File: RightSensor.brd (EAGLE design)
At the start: 17.8 x 19.7 mm, 5 parts, among them X2 CNY70

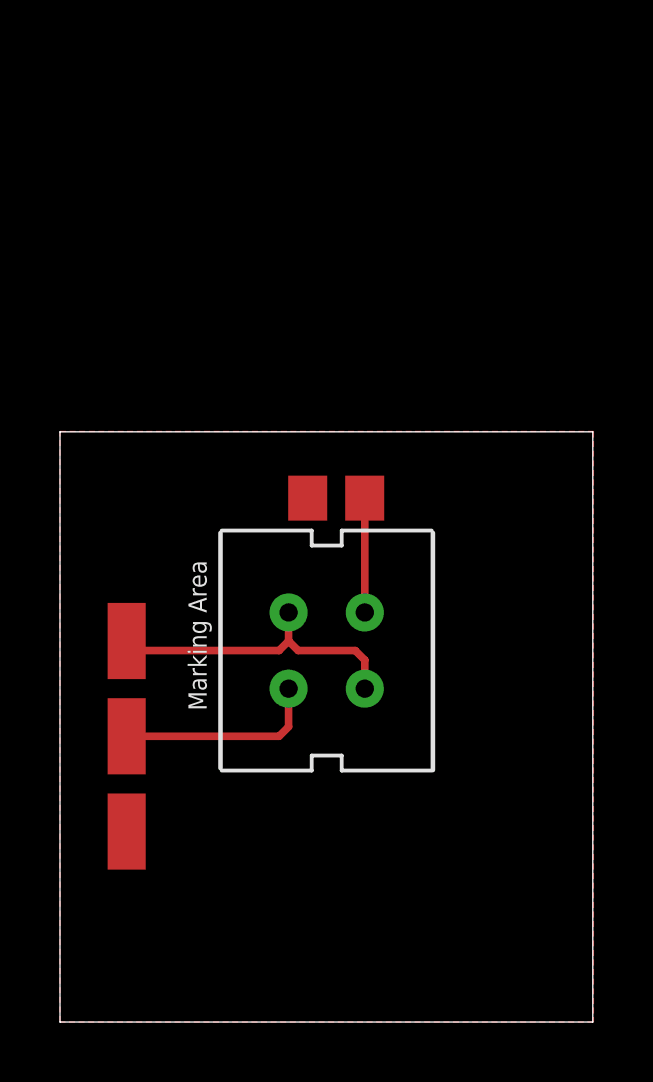
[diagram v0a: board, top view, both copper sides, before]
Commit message: Added code V1
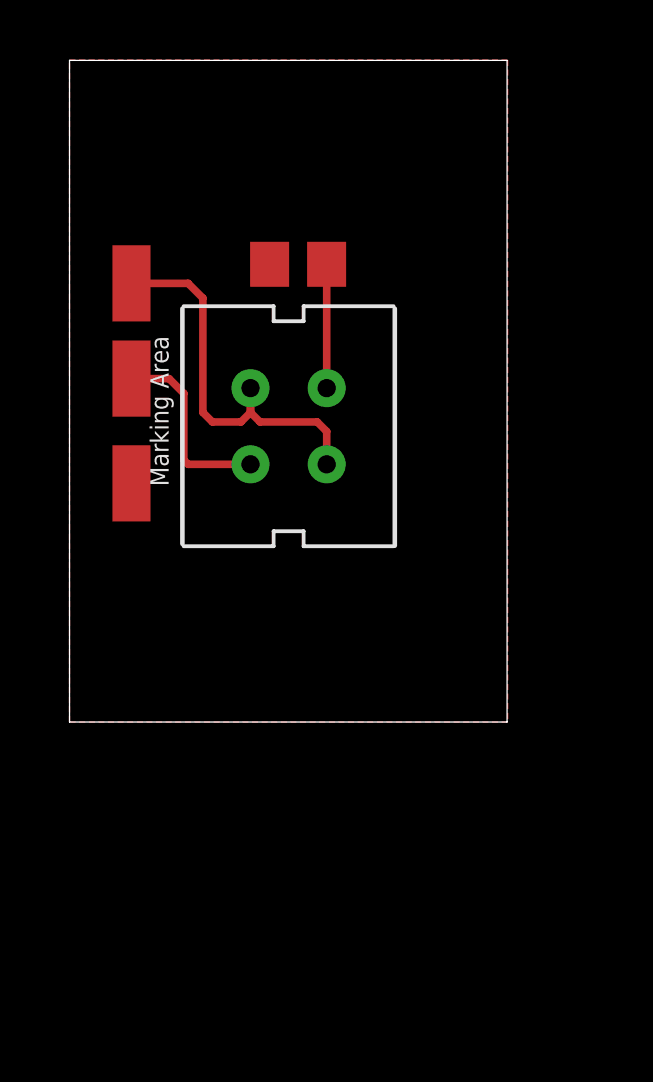
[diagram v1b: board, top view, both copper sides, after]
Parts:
- removed PAD1, PAD2, PAD3: WIREPADSMD1,27-254, wirepad:SMD1,27-2,54
- added PAD4, PAD5, PAD6: WIREPADSMD1,27-254, wirepad:SMD1,27-2,54
- moved R1 7.90 mm to (7.62, 25.3)
- moved X2 7.58 mm to (7.30, 19.9)
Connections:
- net GND: now also PAD6.1; no longer PAD3.1
- net SENSOR: now also PAD5.1; no longer PAD2.1
- net VCC: now also PAD4.1; no longer PAD1.1
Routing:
- net VCC: track 10.4 -> 13.8 mm
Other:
- board size 17.8 x 19.7 mm -> 14.6 x 22.1 mm
